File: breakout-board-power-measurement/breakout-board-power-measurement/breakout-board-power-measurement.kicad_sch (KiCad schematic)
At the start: 62 parts, among them J1 Screw_Terminal_01x04, J2 Conn_01x07, J3 Conn_01x07, J4 Conn_01x02, Q1 NMOS, Q2 NMOS, U1 MCP3911A0-E-SS, U2 Si8641BA-B-IU, U3 LM317_3PinPackage, U4 LM2575-3.3BT, Y1 10M

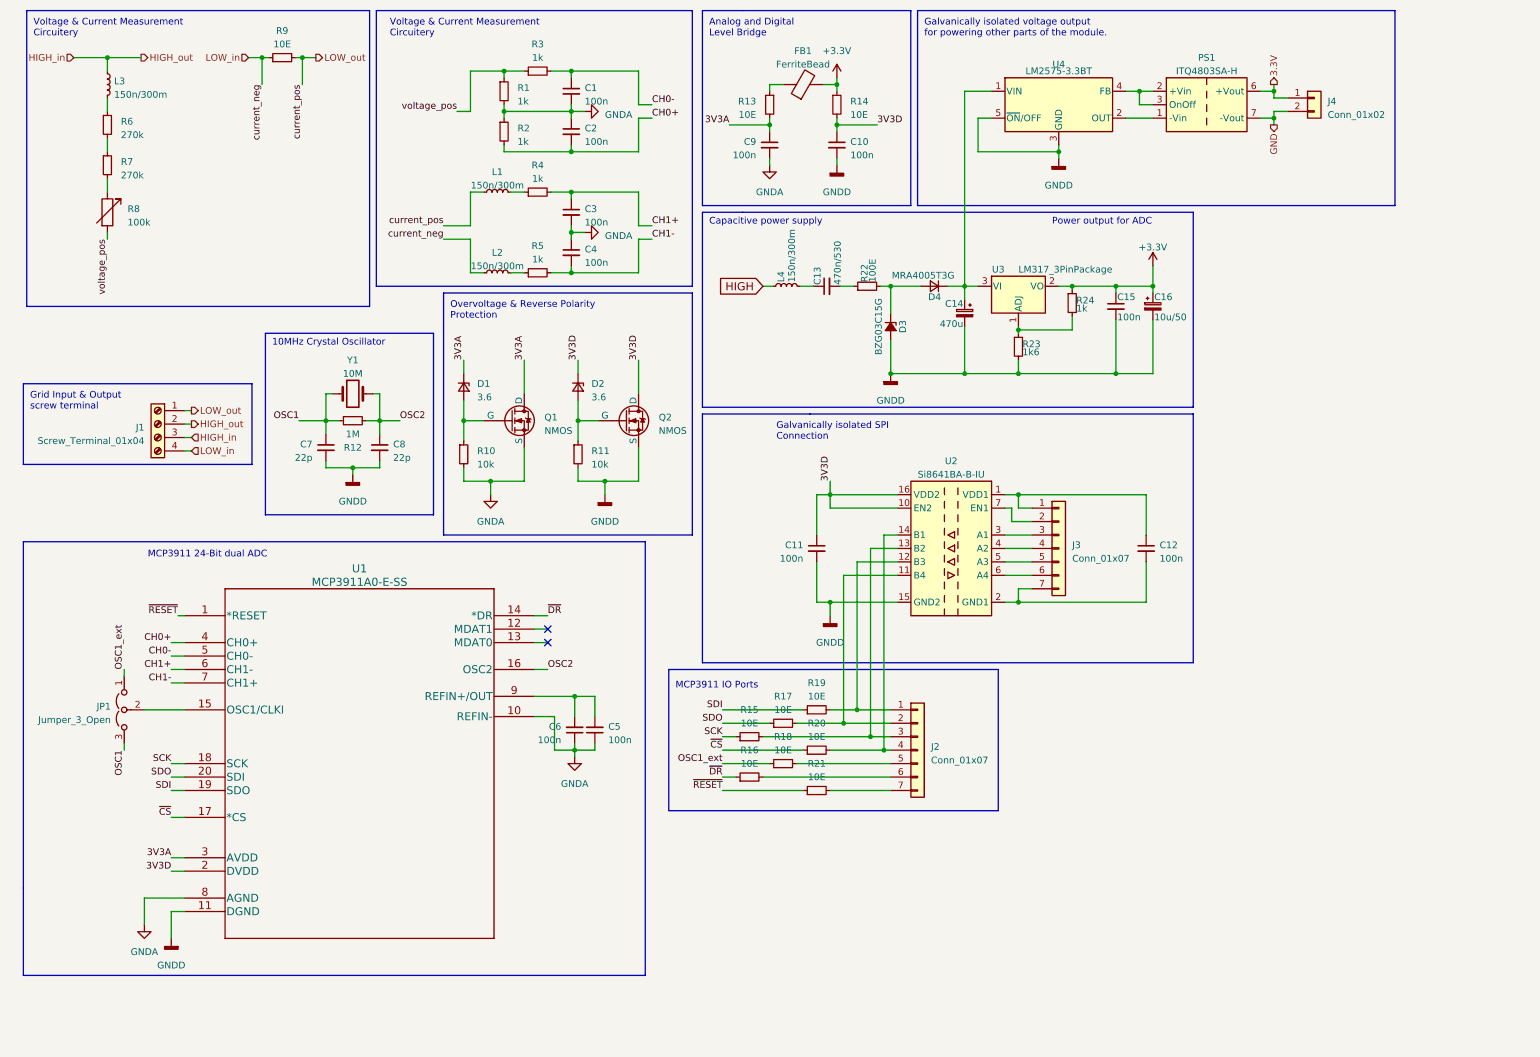
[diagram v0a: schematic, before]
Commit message: Important updates and fine tunings to schematic
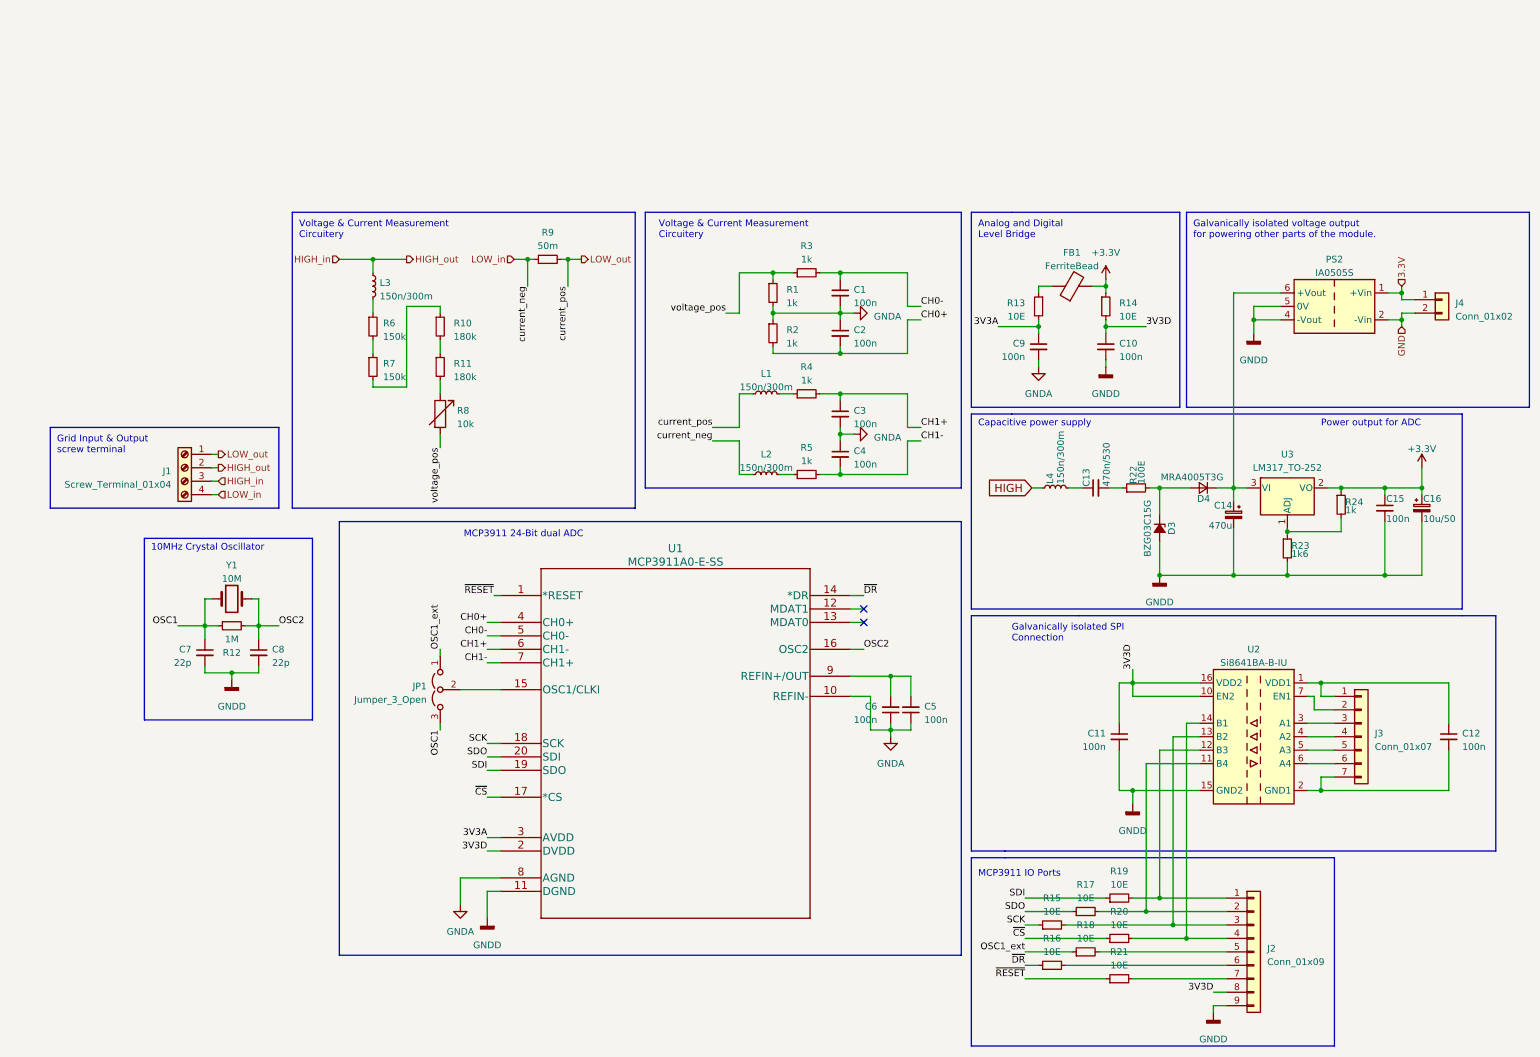
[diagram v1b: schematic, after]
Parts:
- removed D1, D2: 3.6, Diode_SMD:D_1206_3216Metric, symbol Device:D_Zener_Small
- removed PS1: ITQ4803SA-H, Converter_DCDC:Converter_DCDC_XP_POWER-ITQxxxxS-H_THT, symbol Converter_DCDC:ITQ4803SA-H
- removed Q1, Q2: NMOS, Package_TO_SOT_SMD:TO-252-2, symbol Simulation_SPICE:NMOS
- removed U3: LM317_3PinPackage, Package_TO_SOT_SMD:SOT-89-3_Handsoldering, symbol Power-Analyzer-rescue:LM317_3PinPackage
- removed U4: LM2575-3.3BT, Package_TO_SOT_THT:TO-220-5_Vertical, symbol Regulator_Switching:LM2575-3.3BT
- added PS2: IA0505S, Converter_DCDC:Converter_DCDC_XP_POWER-IAxxxxS_THT, symbol Converter_DCDC:IA0505S
- added U3: LM317_TO-252, Package_TO_SOT_SMD:TO-252-2, symbol Regulator_Linear:LM317_TO-252
- J2: value Conn_01x07 -> Conn_01x09; footprint Connector_PinSocket_2.54mm:PinSocket_1x07_P2.54mm_Vertical -> Connector_PinSocket_2.54mm:PinSocket_1x09_P2.54mm_Vertical; symbol Connector_Generic:Conn_01x07 -> Connector_Generic:Conn_01x09
- R10, R11: value 10k -> 180k
- R6, R7: value 270k -> 150k
- R8: value 100k -> 10k
- R9: value 10E -> 50m
- U2: footprint Package_SO:QSOP-16_3.9x4.9mm_P0.635mm -> Package_SO:SOIC-16_3.9x9.9mm_P1.27mm
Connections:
- net +3V3: now also U3.2 (VO)
- net 3.3V: now also PS2.1 (+Vin)
- net 3V3D: now also J2.8 (Pin_8)
- net GND: now also PS2.2 (-Vin)
- net GNDA: no longer R10.2
- net GNDD: now also J2.9 (Pin_9), PS2.4 (-Vout), PS2.5 (0V); no longer R11.2
- net at R10.1: now also R7.2
- net at R11.1: now also R10.2
- net at R8.1: now also R11.2; no longer R7.2
- net at R23.1, R24.2: now also U3.1 (ADJ)
- net at C14.1, D4.1 (K): now also PS2.6 (+Vout), U3.3 (VI)
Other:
- note removed: "Overvoltage & Reverse Polarity Protection"
- moved on the sheet: C1, C10, C11, C12, C13, C14, C15, C16, C2, C3, C4, C5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
